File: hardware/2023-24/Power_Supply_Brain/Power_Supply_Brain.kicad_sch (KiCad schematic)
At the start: 75 parts, among them J1 Conn_02x03_Odd_Even, J2 Conn_01x02, J2 Conn_02x02_Counter_Clockwise, J3 USB_B_Micro, J5 Screw_Terminal_01x06, J6 Conn_02x11_Counter_Clockwise, SW1 SW_MEC_5G, U1 MAX17502G, U2 W25Q128JVS, U3 RP2040, U3 TPSM861252RDXR, U5 NCP1117-5.0_SOT223, Y1 ABLS-12.000MHZ-B4-T

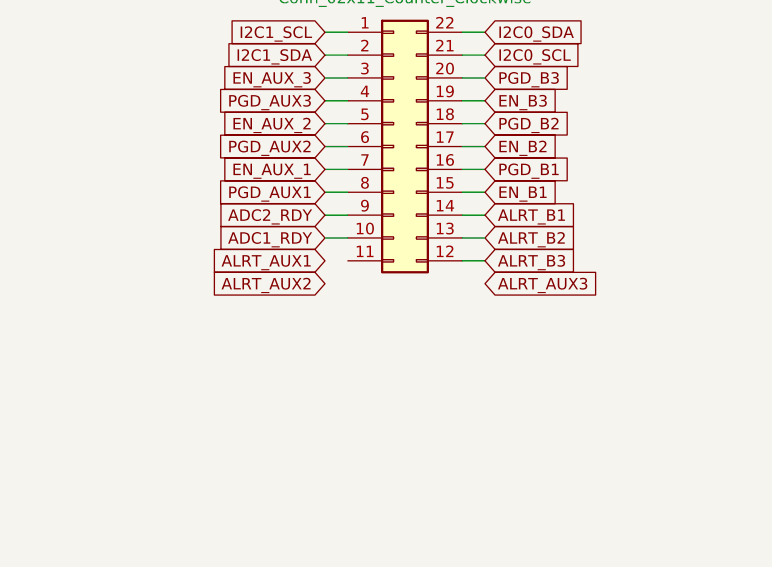
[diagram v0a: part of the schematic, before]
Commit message: Pushing for pre-production review
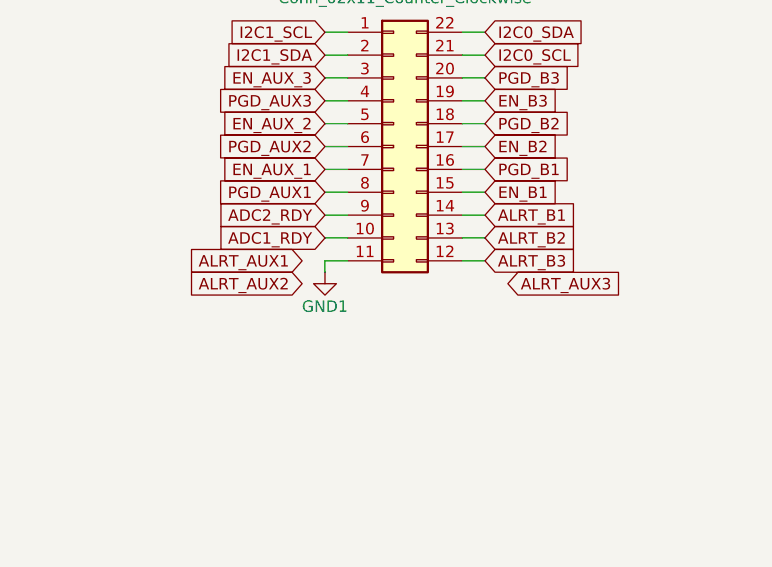
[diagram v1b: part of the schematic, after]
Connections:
- net GND: now also J6.11 (Pin_11)
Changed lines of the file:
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@@
+    (stroke (width 0) (type default))
+  )
+  (wire (pts (xy 356.87 157.48) (xy 356.87 158.75))
     (stroke (width 0) (type default))
   )
@@
   )
   (wire (pts (xy 69.215 136.525) (xy 78.105 136.525))
+    (stroke (width 0) (type default))
+  )
+  (wire (pts (xy 359.41 157.48) (xy 356.87 157.48))
     (stroke (width 0) (type default))
   )
@@
     )
   )
-  (global_label "ALRT_AUX3" (shape input) (at 374.65 160.02 0) (fields_autoplaced)
-    (effects (font (size 1.27 1.27)) (justify left))
-    (property "Intersheetrefs" "${INTERSHEET_REFS}" (at 387.7952 160.02 0)
+  (global_label "ALRT_AUX3" (shape input) (at 377.19 160.02 0) (fields_autoplaced)
+    (effects (font (size 1.27 1.27)) (justify left))
+    (property "Intersheetrefs" "${INTERSHEET_REFS}" (at 390.3352 160.02 0)
       (effects (font (size 1.27 1.27)) (justify left) hide)
     )
@@
     )
   )
-  (global_label "ALRT_AUX1" (shape input) (at 356.87 157.48 180) (fields_autoplaced)
-    (effects (font (size 1.27 1.27)) (justify right))
-    (property "Intersheetrefs" "${INTERSHEET_REFS}" (at 343.7248 157.48 0)
+  (global_label "ALRT_AUX1" (shape input) (at 354.33 157.48 180) (fields_autoplaced)
+    (effects (font (size 1.27 1.27)) (justify right))
+    (property "Intersheetrefs" "${INTERSHEET_REFS}" (at 341.1848 157.48 0)
       (effects (font (size 1.27 1.27)) (justify right) hide)
     )
@@
     )
   )
-  (global_label "ALRT_AUX2" (shape input) (at 356.87 160.02 180) (fields_autoplaced)
-    (effects (font (size 1.27 1.27)) (justify right))
-    (property "Intersheetrefs" "${INTERSHEET_REFS}" (at 343.7248 160.02 0)
+  (global_label "ALRT_AUX2" (shape input) (at 354.33 160.02 180) (fields_autoplaced)
+    (effects (font (size 1.27 1.27)) (justify right))
+    (property "Intersheetrefs" "${INTERSHEET_REFS}" (at 341.1848 160.02 0)
       (effects (font (size 1.27 1.27)) (justify right) hide)
     )
@@
         )
       )
+    )
+  )
+  (symbol (lib_id "power:GND1") (at 356.87 158.75 0) (unit 1)
+    (in_bom yes) (on_board yes) (dnp no)
+    (property "Reference" "#PWR063" (at 356.87 165.1 0)
+      (effects (font (size 1.27 1.27)) hide)
+    )
+    (property "Value" "GND1" (at 359.41 162.56 0)
+      (effects (font (size 1.27 1.27)) (justify right))
+    )
+    (property "Footprint" "" (at 356.87 158.75 0)
+      (effects (font (size 1.27 1.27)) hide)
+    )
+    (property "Datasheet" "" (at 356.87 158.75 0)
+      (effects (font (size 1.27 1.27)) hide)
+    )
+    (pin "1")
+    (instances
+      (project "Power_Supply_Brain"
+        (path "/3e3c1858-5f82-4870-a9c4-db8f7fe14a45"
+          (reference "#PWR063") (unit 1)
+        )
+      )
+      (project "2023-24_Power_Supply"
+        (path "/9d08c113-56e0-4c7c-90b4-94c67f8b2e1a"
+          (reference "#PWR033") (unit 1)
+        )
+      )
